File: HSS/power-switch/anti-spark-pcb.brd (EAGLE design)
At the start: 31.4 x 18 mm, 9 parts

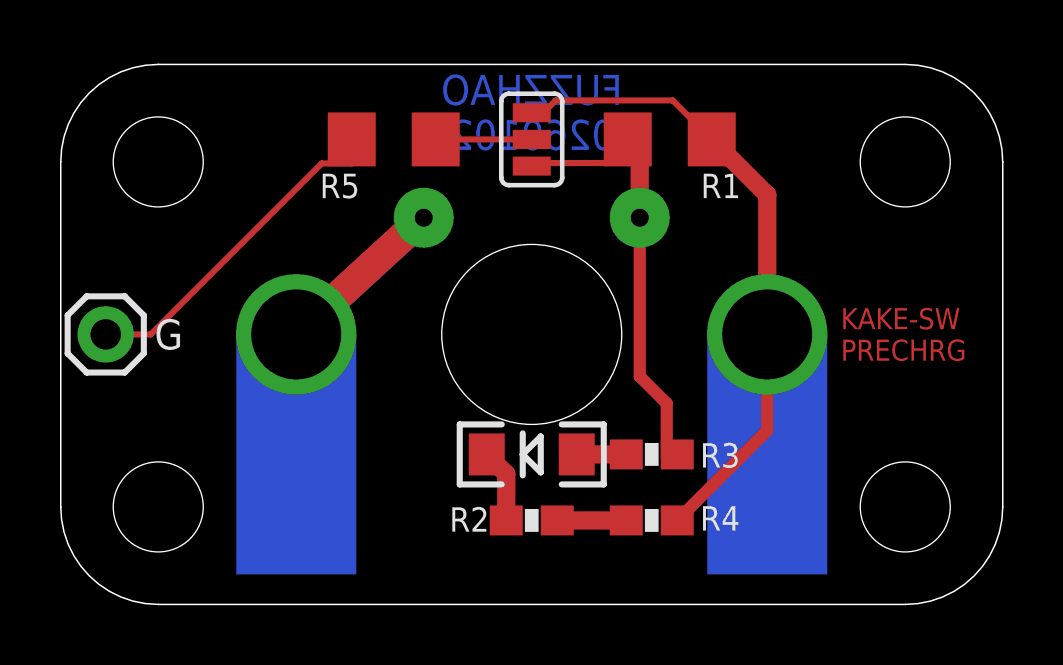
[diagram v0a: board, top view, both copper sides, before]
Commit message: uncommitted PCBs
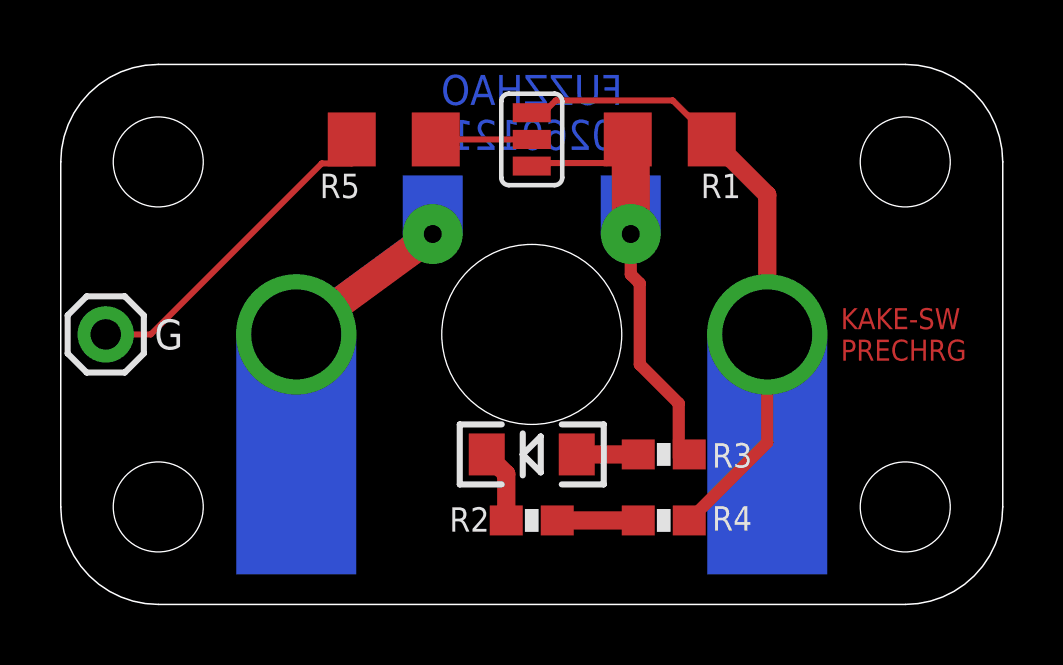
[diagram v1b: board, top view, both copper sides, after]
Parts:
- moved R3 0.40 mm to (20.1, 5.00)
- moved R4 0.40 mm to (20.1, 2.80)
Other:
- board text added: "FUZZHAO 20260121A"
- board text removed: "FUZZHAO 20260102A"
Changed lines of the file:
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@@
 <grid distance="0.1" unitdist="mm" unit="mm" style="lines" multiple="10" display="yes" altdistance="0.05" altunitdist="mm" altunit="mm"/>
 <layers>
-<layer number="1" name="Top" color="4" fill="1" visible="yes" active="yes"/>
+<layer number="1" name="Top" color="4" fill="1" visible="no" active="yes"/>
 <layer number="2" name="Route2" color="1" fill="3" visible="no" active="no"/>
 <layer number="3" name="Route3" color="4" fill="3" visible="no" active="no"/>
@@
 PRECHRG</text>
 <text x="15.7" y="16.4" size="1" layer="16" font="vector" ratio="12" rot="MR0" align="center">FUZZHAO
-20260102A</text>
+20260121A</text>
 <text x="3.6" y="9" size="1" layer="25" font="vector" ratio="12" align="center">G</text>
+<text x="15.7" y="16.4" size="1" layer="30" font="vector" ratio="12" rot="MR0" align="center">FUZZHAO
+20260121A</text>
 </plain>
 <attributes>
@@
 <attribute name="NAME" x="14.289" y="3.238" size="0.8128" layer="25" font="vector" rot="R180"/>
 </element>
-<element name="R3" library="anti-spark-pcb" package="0603-RES" value="0ZCM0001FF2G" x="19.7" y="5" smashed="yes" rot="R180">
-<attribute name="NAME" x="21.311" y="4.562" size="0.8128" layer="25" font="vector"/>
-</element>
-<element name="R4" library="anti-spark-pcb" package="0603-RES" value="" x="19.7" y="2.8" smashed="yes">
-<attribute name="NAME" x="21.311" y="2.462" size="0.8128" layer="25" font="vector"/>
-<attribute name="VALUE" x="18.684" y="1.657" size="0.4064" layer="27" font="vector"/>
+<element name="R3" library="anti-spark-pcb" package="0603-RES" value="0ZCM0001FF2G" x="20.1" y="5" smashed="yes" rot="R180">
+<attribute name="NAME" x="21.711" y="4.562" size="0.8128" layer="25" font="vector"/>
+</element>
+<element name="R4" library="anti-spark-pcb" package="0603-RES" value="" x="20.1" y="2.8" smashed="yes">
+<attribute name="NAME" x="21.711" y="2.462" size="0.8128" layer="25" font="vector"/>
+<attribute name="VALUE" x="19.084" y="1.657" size="0.4064" layer="27" font="vector"/>
 </element>
 <element name="LED1" library="anti-spark-pcb" package="LED-1206" value="" x="15.7" y="5" smashed="yes" rot="R180">
@@
 <contactref element="PCB1" pad="B2"/>
 <contactref element="R1" pad="2"/>
-<wire x1="19.3" y1="12.89" x2="19.3" y2="15.5" width="0.6096" layer="1"/>
 <wire x1="19.3" y1="15.5" x2="18.9" y2="15.5" width="0.6096" layer="1"/>
 <contactref element="R3" pad="1"/>
-<wire x1="19.3" y1="7.6" x2="19.3" y2="12.89" width="0.4064" layer="1"/>
 <contactref element="SJ1" pad="3"/>
 <wire x1="15.7" y1="14.611" x2="15.8" y2="14.711" width="0.2032" layer="1"/>
 <wire x1="15.8" y1="14.711" x2="18.211" y2="14.711" width="0.2032" layer="1"/>
 <wire x1="18.211" y1="14.711" x2="18.9" y2="15.5" width="0.2032" layer="1"/>
-<wire x1="19.3" y1="7.6" x2="20.2" y2="6.7" width="0.4064" layer="1"/>
-<wire x1="20.2" y1="6.7" x2="20.2" y2="4.9" width="0.4064" layer="1"/>
-<wire x1="20.2" y1="4.9" x2="20.55" y2="5" width="0.2032" layer="1"/>
+<wire x1="19.3" y1="8" x2="20.6" y2="6.7" width="0.4064" layer="1"/>
+<wire x1="20.6" y1="6.7" x2="20.6" y2="4.9" width="0.4064" layer="1"/>
+<wire x1="20.6" y1="4.9" x2="20.95" y2="5" width="0.2032" layer="1"/>
+<wire x1="19" y1="12.347" x2="19" y2="15.4" width="1.27" layer="1"/>
+<wire x1="19" y1="15.4" x2="18.9" y2="15.5" width="1.27" layer="1"/>
+<wire x1="19.3" y1="8" x2="19.3" y2="10.7" width="0.4064" layer="1"/>
+<wire x1="19.3" y1="10.7" x2="19" y2="11" width="0.4064" layer="1"/>
+<wire x1="19" y1="11" x2="19" y2="12.347" width="0.4064" layer="1"/>
 </signal>
 <signal name="N$2">
@@
 <wire x1="23.55" y1="13.65" x2="23.55" y2="9" width="0.6096" layer="1"/>
 <contactref element="R4" pad="2"/>
-<wire x1="20.55" y1="2.8" x2="23.55" y2="5.8" width="0.4064" layer="1"/>
-<wire x1="23.55" y1="5.8" x2="23.55" y2="9" width="0.4064" layer="1"/>
+<wire x1="20.95" y1="2.8" x2="23.55" y2="5.4" width="0.4064" layer="1"/>
+<wire x1="23.55" y1="5.4" x2="23.55" y2="9" width="0.4064" layer="1"/>
 <contactref element="SJ1" pad="1"/>
 <wire x1="21.7" y1="15.5" x2="20.4" y2="16.8" width="0.2032" layer="1"/>
@@
 <contactref element="PCB1" pad="A1"/>
 <contactref element="PCB1" pad="B1"/>
-<wire x1="7.85" y1="9" x2="12.1" y2="12.89" width="1" layer="16"/>
+<wire x1="7.85" y1="9" x2="12.4" y2="12.347" width="1" layer="16"/>
 </signal>
 <signal name="N$4">
-<wire x1="7.85" y1="9" x2="12.1" y2="12.9" width="1" layer="1"/>
+<wire x1="7.85" y1="9" x2="12.5" y2="12.4" width="1.016" layer="1"/>
 </signal>
 <signal name="N$5">
 <contactref element="R3" pad="2"/>
 <contactref element="LED1" pad="A"/>
-<wire x1="17.2" y1="5" x2="18.85" y2="5" width="0.6096" layer="1"/>
+<wire x1="17.2" y1="5" x2="19.25" y2="5" width="0.6096" layer="1"/>
 </signal>
 <signal name="N$6">
 <contactref element="R4" pad="1"/>
 <contactref element="R2" pad="2"/>
-<wire x1="16.55" y1="2.8" x2="18.85" y2="2.8" width="0.6096" layer="1"/>
+<wire x1="16.55" y1="2.8" x2="19.25" y2="2.8" width="0.6096" layer="1"/>
 </signal>
 <signal name="N$7">
